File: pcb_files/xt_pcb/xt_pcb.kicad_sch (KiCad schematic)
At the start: 15 parts, among them J1 JST, SW1 RST, SW2 RST, U1 STM32F072C8Tx, U2 XC6206PxxxMR-Regulator_Linear

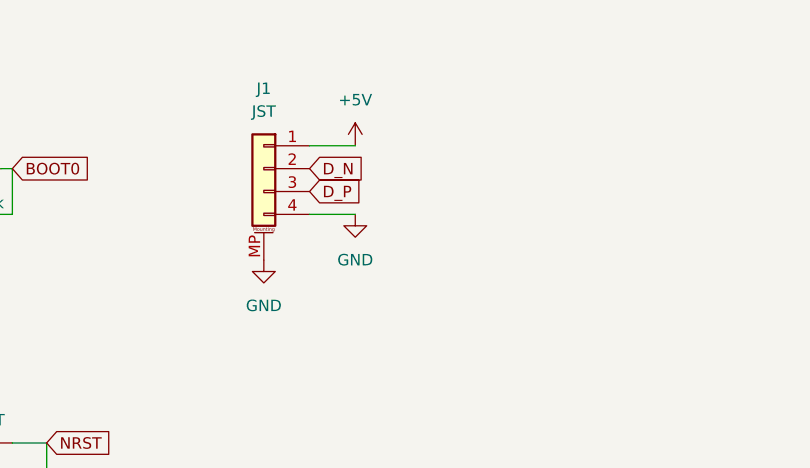
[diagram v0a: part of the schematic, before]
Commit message: fixes
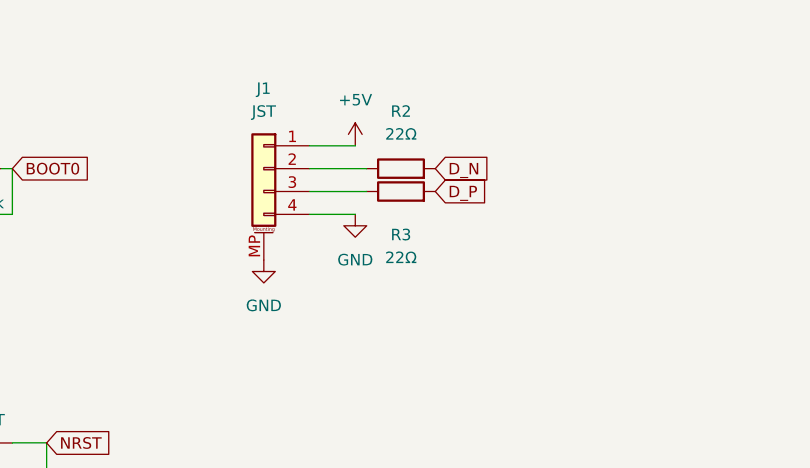
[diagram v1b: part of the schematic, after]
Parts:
- added R2, R3: 22Ω, Capacitor_SMD:C_0402_1005Metric, symbol Device:R
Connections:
- net D_N: now also R2.2; no longer J1.2 (Pin_2)
- net D_P: now also R3.2; no longer J1.3 (Pin_3)
- new net: J1.2 (Pin_2), R2.1
- new net: J1.3 (Pin_3), R3.1
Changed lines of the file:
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@@
+	(wire
+		(pts
+			(xy 157.48 35.56) (xy 151.13 35.56)
+		)
+		(stroke
+			(width 0)
+			(type default)
+		)
+	)
 	(wire
 		(pts
@@
 	(wire
 		(pts
+			(xy 157.48 38.1) (xy 151.13 38.1)
+		)
+		(stroke
+			(width 0)
+			(type default)
+		)
+	)
+	(wire
+		(pts
 			(xy 173.99 107.95) (xy 182.88 107.95)
 		)
@@
 	(global_label "D_P"
 		(shape input)
-		(at 151.13 38.1 0)
-		(fields_autoplaced yes)
-		(effects
-			(font
-				(size 1.27 1.27)
-			)
-			(justify left)
-		)
-		(property "Intersheetrefs" "${INTERSHEET_REFS}"
-			(at 157.0507 38.1794 0)
+		(at 165.1 38.1 0)
+		(fields_autoplaced yes)
+		(effects
+			(font
+				(size 1.27 1.27)
+			)
+			(justify left)
+		)
+		(property "Intersheetrefs" "${INTERSHEET_REFS}"
+			(at 171.0207 38.1794 0)
 			(effects
 				(font
@@
 	(global_label "D_N"
 		(shape input)
-		(at 151.13 35.56 0)
-		(fields_autoplaced yes)
-		(effects
-			(font
-				(size 1.27 1.27)
-			)
-			(justify left)
-		)
-		(property "Intersheetrefs" "${INTERSHEET_REFS}"
-			(at 157.1112 35.6394 0)
+		(at 165.1 35.56 0)
+		(fields_autoplaced yes)
+		(effects
+			(font
+				(size 1.27 1.27)
+			)
+			(justify left)
+		)
+		(property "Intersheetrefs" "${INTERSHEET_REFS}"
+			(at 171.0812 35.6394 0)
 			(effects
 				(font
@@
 	)
 	(symbol
+		(lib_id "Device:R")
+		(at 161.29 35.56 90)
+		(unit 1)
+		(exclude_from_sim no)
+		(in_bom yes)
+		(on_board yes)
+		(dnp no)
+		(fields_autoplaced yes)
+		(property "Reference" "R2"
+			(at 161.29 29.21 90)
+			(effects
+				(font
+					(size 1.27 1.27)
+				)
+			)
+		)
+		(property "Value" "22Ω"
+			(at 161.29 31.75 90)
+			(effects
+				(font
+					(size 1.27 1.27)
+				)
+			)
+		)
+		(property "Footprint" "Capacitor_SMD:C_0402_1005Metric"
+			(at 161.29 37.338 90)
+			(effects
+				(font
+					(size 1.27 1.27)
+				)
+				(hide yes)
+			)
+		)
+		(property "Datasheet" "~"
+			(at 161.29 35.56 0)
+			(effects
+				(font
+					(size 1.27 1.27)
+				)
+				(hide yes)
+			)
+		)
+		(property "Description" "Resistor"
+			(at 161.29 35.56 0)
+			(effects
+				(font
+					(size 1.27 1.27)
+				)
+				(hide yes)
+			)
+		)
+		(pin "2"
+		)
+		(pin "1"
+		)
+		(instances
+			(project ""
+				(path "/0d76ce34-a40d-405c-820f-030fec8e9950"
+					(reference "R2")
+					(unit 1)
+				)
+			)
+		)
+	)
+	(symbol
 		(lib_id "Device:C_Small")
 		(at 105.41 107.95 180)
@@
 					(unit 1)
 				)
+			)
+		)
+	)
+	(symbol
+		(lib_id "Device:R")
+		(at 161.29 38.1 90)
+		(unit 1)
+		(exclude_from_sim no)
+		(in_bom yes)
+		(on_board yes)
+		(dnp no)
+		(property "Reference" "R3"
+			(at 161.29 42.926 90)
+			(effects
+				(font
+					(size 1.27 1.27)
+				)
+			)
+		)
+		(property "Value" "22Ω"
+			(at 161.29 45.466 90)
+			(effects
+				(font
+					(size 1.27 1.27)
+				)
+			)
+		)
+		(property "Footprint" "Capacitor_SMD:C_0402_1005Metric"
+			(at 161.29 39.878 90)
+			(effects
+				(font
+					(size 1.27 1.27)
+				)
+				(hide yes)
+			)
+		)
+		(property "Datasheet" "~"
+			(at 161.29 38.1 0)
+			(effects
+				(font
+					(size 1.27 1.27)
+				)
+				(hide yes)
+			)
+		)
+		(property "Description" "Resistor"
+			(at 161.29 38.1 0)
+			(effects
+				(font
+					(size 1.27 1.27)
+				)
+				(hide yes)
+			)
+		)
+		(pin "2"
+		)
+		(pin "1"
+		)
+		(instances
+			(project ""
+				(path "/0d76ce34-a40d-405c-820f-030fec8e9950"
+					(reference "R3")
+					(unit 1)
+				)

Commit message: 0603 handsolder
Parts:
- C2: footprint Capacitor_SMD:C_0402_1005Metric -> Capacitor_SMD:C_0603_1608Metric_Pad1.08x0.95mm_HandSolder
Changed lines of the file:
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@@
 			)
 		)
-		(property "Footprint" "Capacitor_SMD:C_0402_1005Metric"
+		(property "Footprint" "Capacitor_SMD:C_0603_1608Metric_Pad1.08x0.95mm_HandSolder"
 			(at 113.03 71.12 0)
 			(effects

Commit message: updated lcsc information
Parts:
- C4: LCSC C52923 -> C23733
- J1: LCSC C145956 -> C588524
- R1: LCSC (none) -> C25744
- R2, R3: LCSC (none) -> C25092
- SW1, SW2: LCSC (none) -> C139779
- U1: LCSC (none) -> C80488
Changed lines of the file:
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@@
 		)
 		(property "LCSC" "C307331"
-			(at 113.03 71.12 0)
+			(at 113.03 71.12 90)
 			(effects
 				(font
@@
 			)
 		)
+		(property "LCSC" "C25092"
+			(at 161.29 35.56 90)
+			(effects
+				(font
+					(size 1.27 1.27)
+				)
+				(hide yes)
+			)
+		)
 		(pin "2"
 		)
@@
 			)
 		)
+		(property "LCSC" "C25092"
+			(at 161.29 38.1 90)
+			(effects
+				(font
+					(size 1.27 1.27)
+				)
+				(hide yes)
+			)
+		)
 		(pin "2"
 		)
@@
 			)
 		)
-		(property "LCSC" "C52923"
+		(property "LCSC" "C23733"
 			(at 148.59 104.14 0)
 			(effects
@@
 			)
 		)
-		(property "LCSC" ""
+		(property "LCSC" "C139779"
 			(at 113.03 66.04 0)
 			(effects
@@
 			)
 		)
-		(property "LCSC" "C145956"
+		(property "LCSC" "C588524"
 			(at 146.05 35.56 0)
 			(effects
@@
 			)
 		)
+		(property "LCSC" "C80488"
+			(at 59.69 73.66 0)
+			(effects
+				(font
+					(size 1.27 1.27)
+				)
+				(hide yes)
+			)
+		)
 		(pin "1"
 		)
@@
 			)
 		)
-		(property "LCSC" ""
+		(property "LCSC" "C139779"
 			(at 111.76 35.56 0)
 			(effects
@@
 			)
 		)
+		(property "LCSC" "C25744"
+			(at 111.76 40.64 90)
+			(effects
+				(font
+					(size 1.27 1.27)
+				)
+				(hide yes)
+			)
+		)
